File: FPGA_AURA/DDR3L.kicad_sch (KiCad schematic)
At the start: 42 parts, among them U500 MT41K128M16JT-125_IT_K

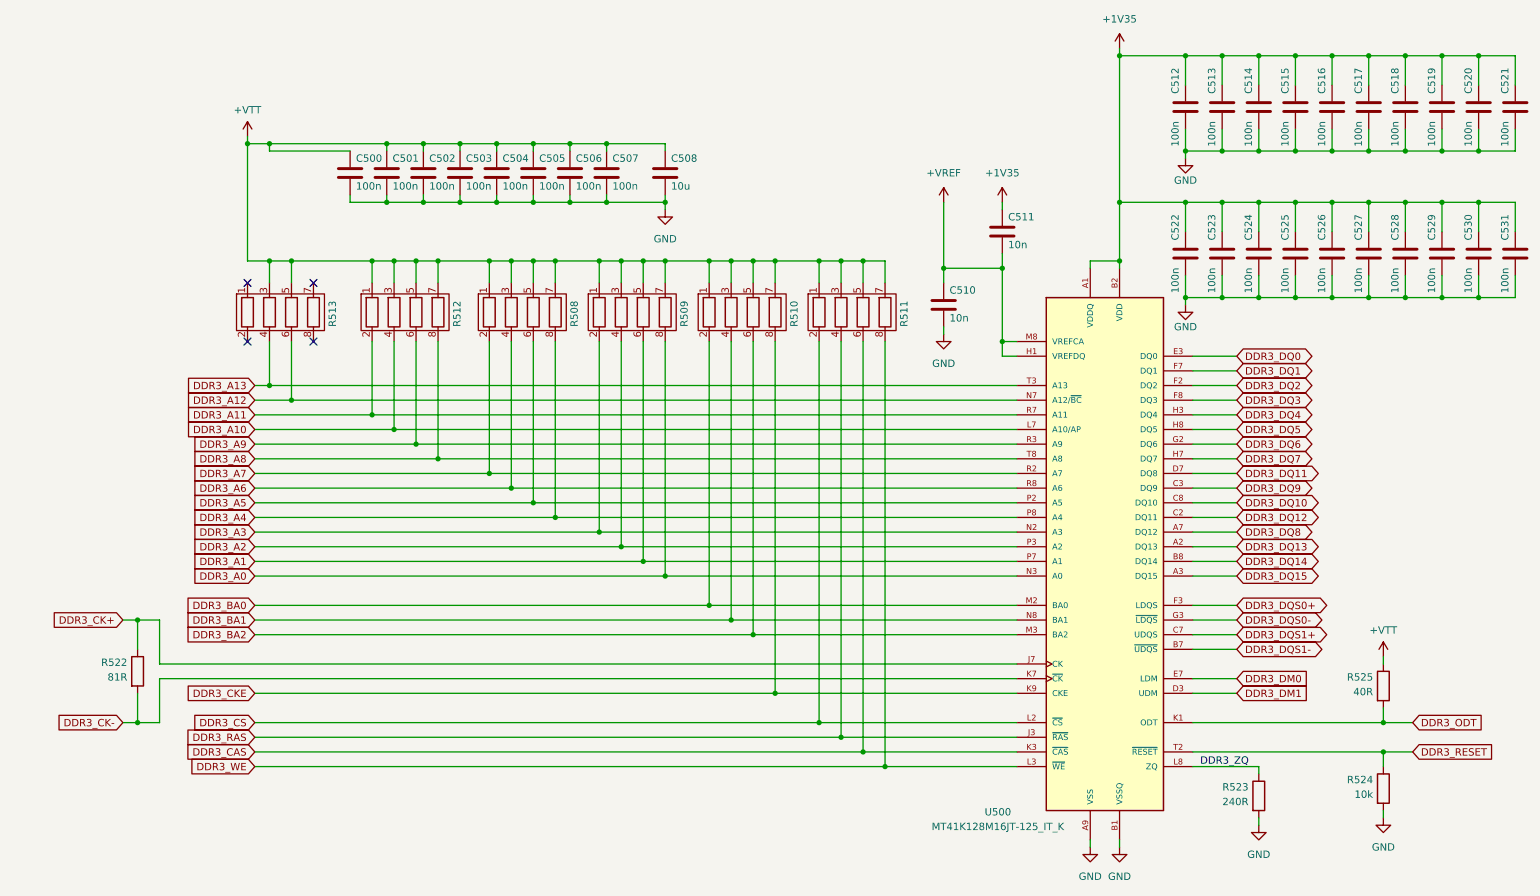
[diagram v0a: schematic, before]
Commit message: Continuing the FTDI
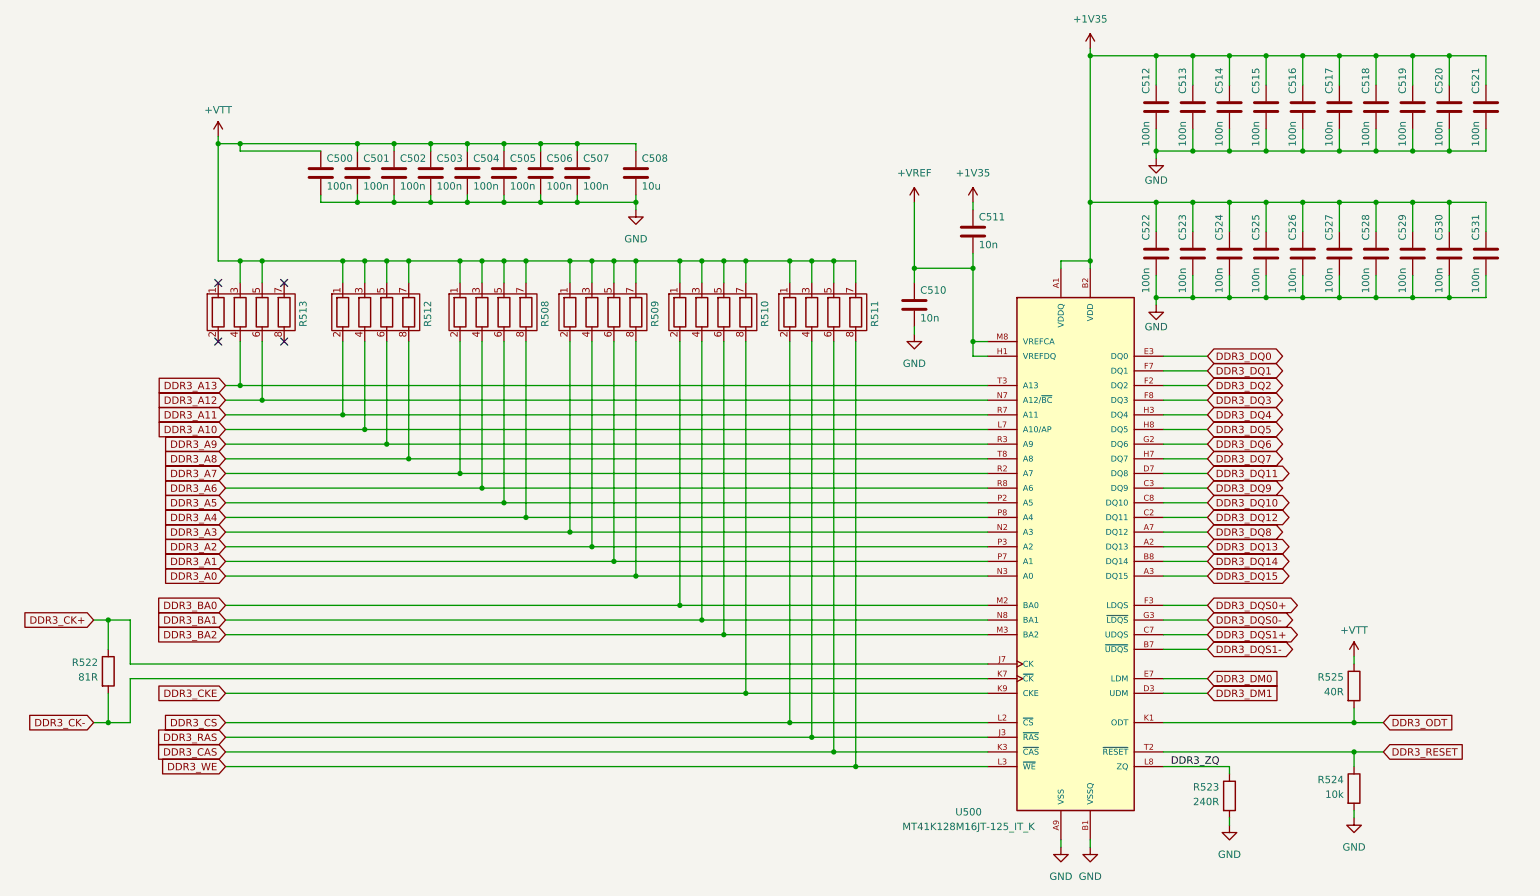
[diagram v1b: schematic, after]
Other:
- moved on the sheet: C500, C501, C502, C503, C504, C505, C506, C507, C508, C510, C511, C512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
